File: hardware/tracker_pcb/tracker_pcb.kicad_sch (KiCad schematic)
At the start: 37 parts, among them IC1 THVD1426DRLR, IC2 DRV8244HQRYJRQ1, J1 256-406, U1 DRV8243HQRXYRQ1, U2 DRV8243HQRXYRQ1, U3 TPS62933FDRLR, U4 ESP32C6_SEEED, X1 256-402

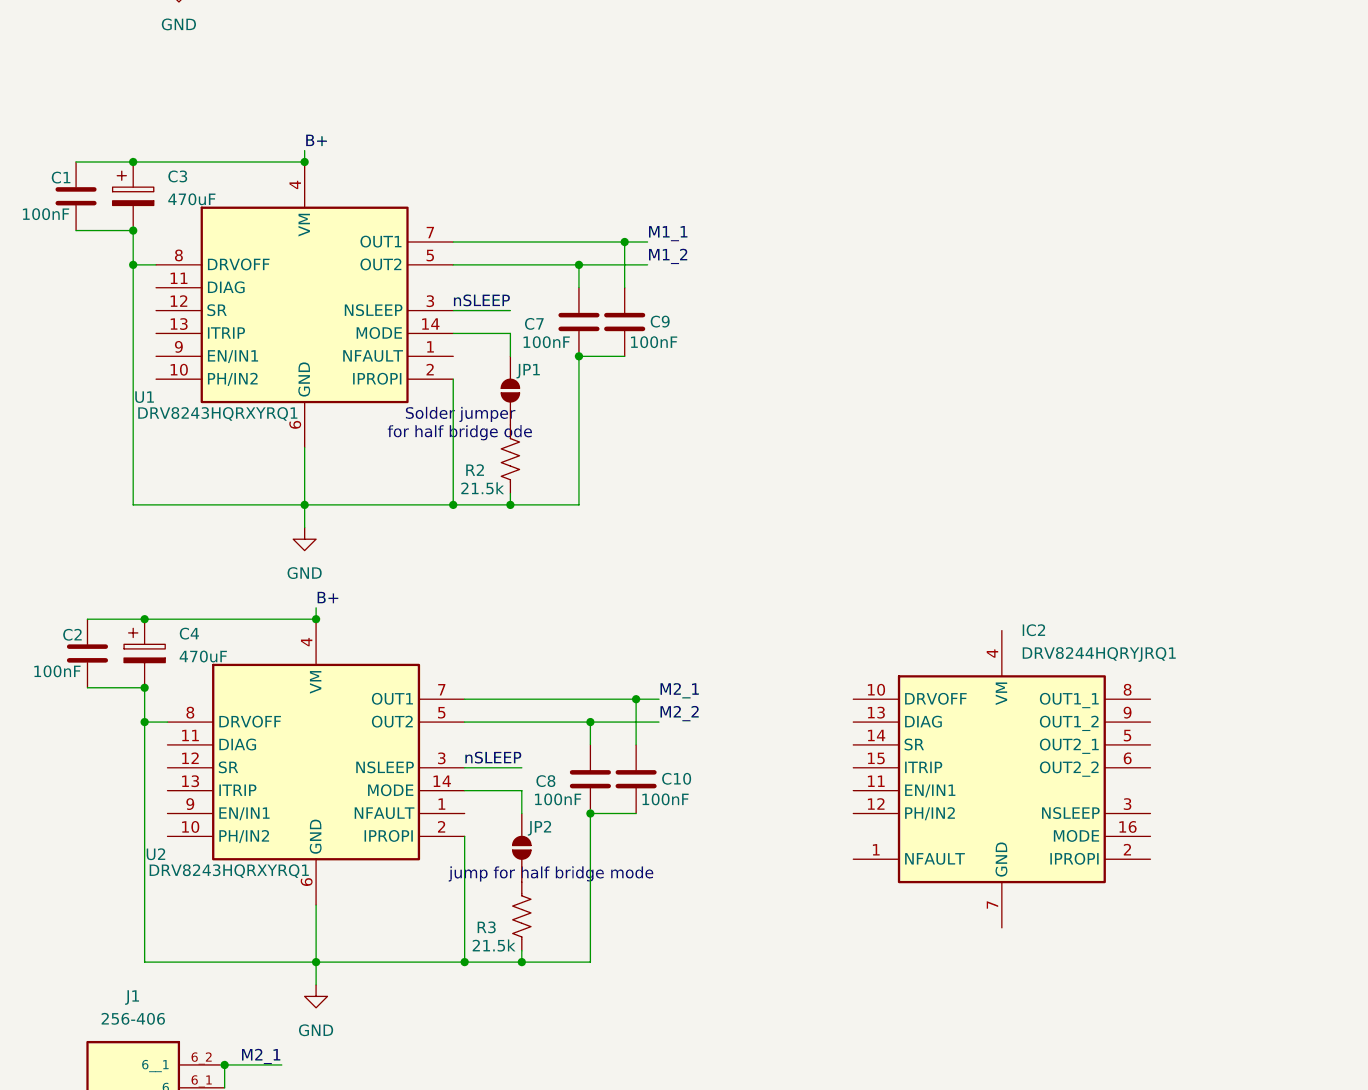
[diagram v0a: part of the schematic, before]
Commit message: wip
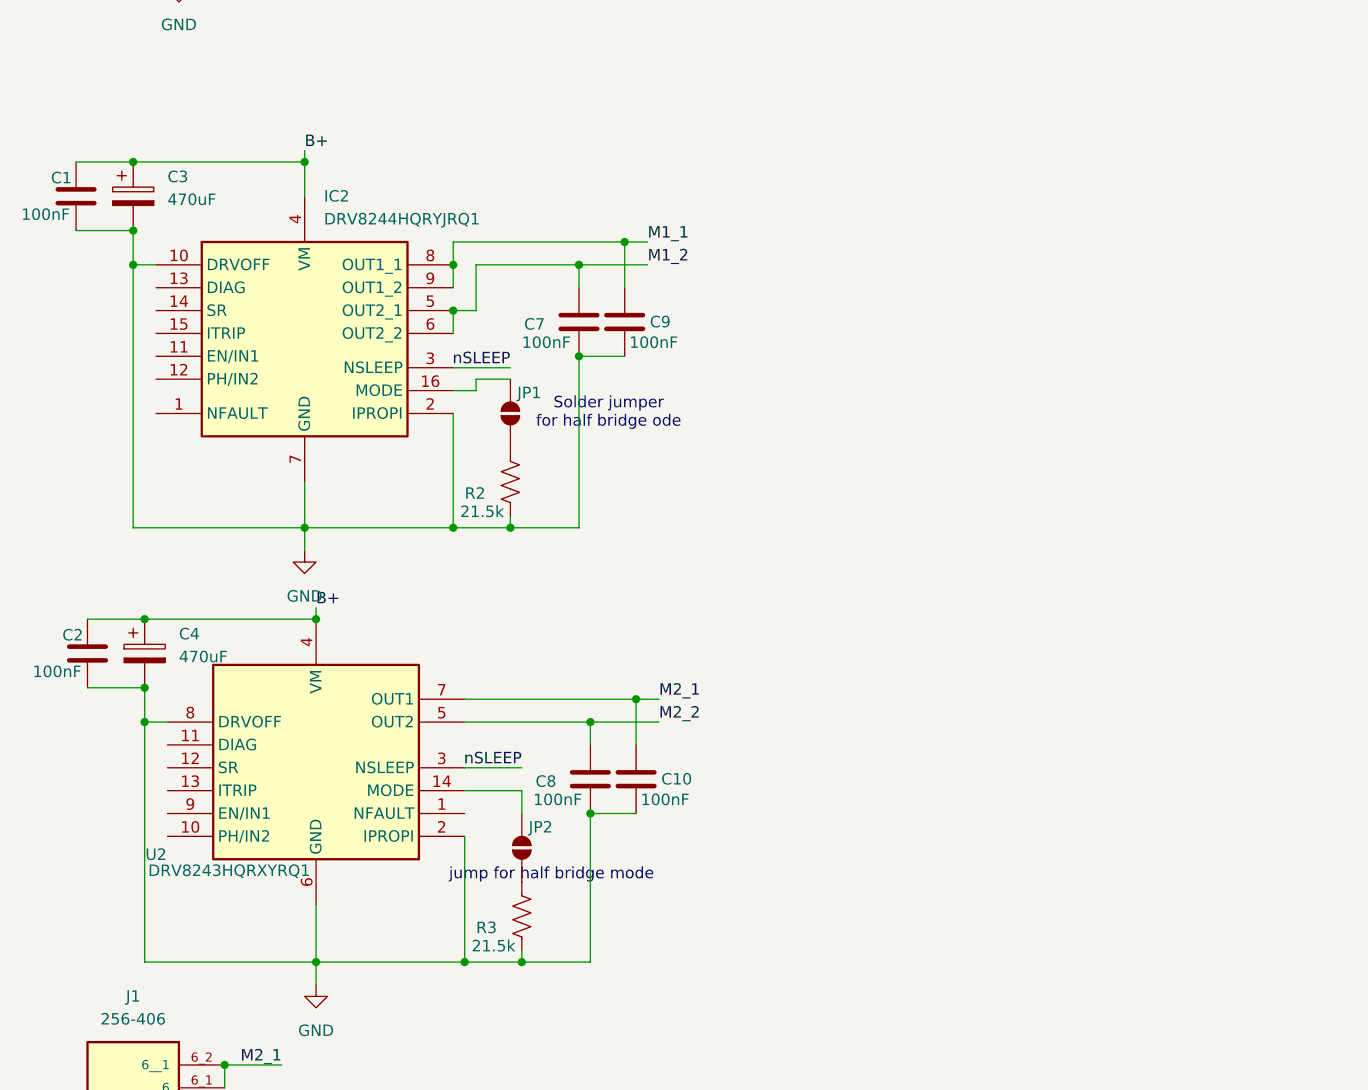
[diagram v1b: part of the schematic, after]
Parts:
- removed U1: DRV8243HQRXYRQ1, DRV8243HQRXYRQ1, symbol symbol:DRV8243HQRXYRQ1
- IC2: footprint footprint:DRV8244HQRYJRQ1 -> DRV8244HQRYJRQ1
- L1: footprint footprint:IND-SMD_L12.3-W12.3 -> Inductor_SMD:L_10.4x10.4_H4.8
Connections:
- net B+: now also IC2.4 (VM)
- net GND: now also IC2.10 (DRVOFF), IC2.2 (IPROPI), IC2.7 (GND)
- net M1_1: now also IC2.8 (OUT1_1), IC2.9 (OUT1_2)
- net M1_2: now also IC2.5 (OUT2_1), IC2.6 (OUT2_2)
- net nSLEEP: now also IC2.3 (NSLEEP)
- net at JP1.2 (B): now also IC2.16 (MODE)
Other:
- moved on the sheet: IC2, JP1, R2
